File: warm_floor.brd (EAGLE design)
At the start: 52 x 40 mm, 31 parts, among them K1 G2R, Q1 BSS123, T1 BC847, T2 BC847, T3 BC847, X1 53047-04, X3 DG3XX-03-3.5, X4 DG3XX-02-3.5

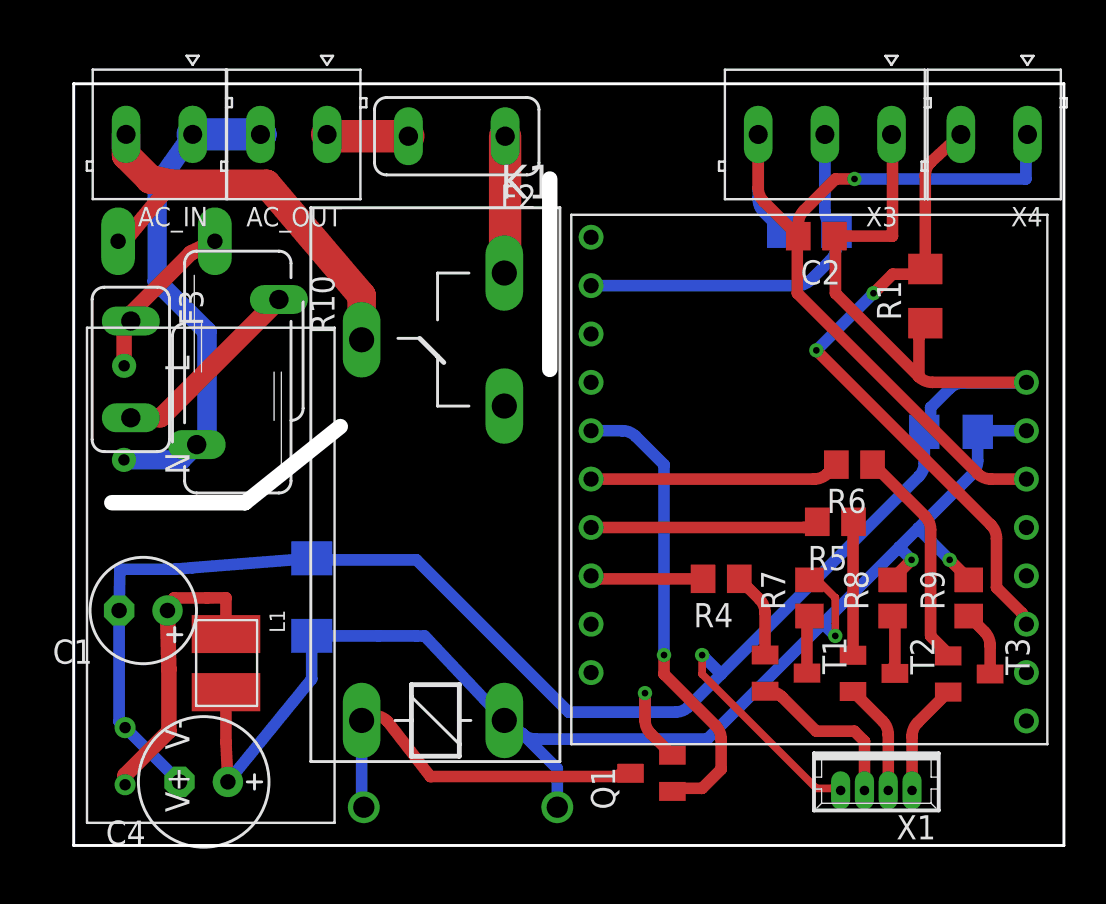
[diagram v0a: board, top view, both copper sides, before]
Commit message: Last G2R version
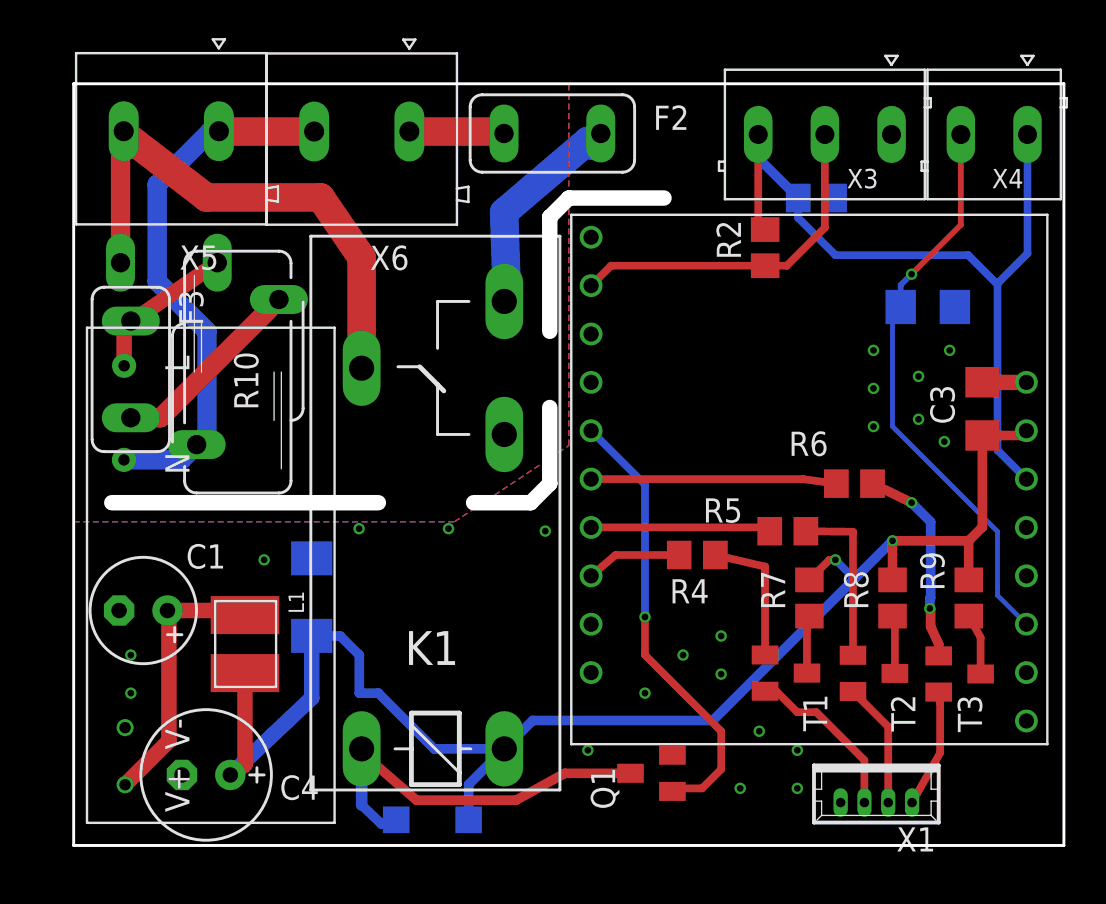
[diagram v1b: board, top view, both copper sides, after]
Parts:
- removed AC_IN, AC_OUT: DG3XX-02-3.5, degson:DG350-3.5-02P
- added X5, X6: DG3XX-025.0, degson:DG300-5.0-02P
- D1: value 1N4004 -> (none); device diode:DO41-10 -> diode:SOD123
- D2: value SMBJ20A -> SMBJ15A
- F1: value (none) -> FUSETE5; device fuse:TR5 -> fuse:TE5
- R2: device resistor:R1206 -> rcl:R0805
- moved F2 5.02 mm to (25.1, 37.4)
- moved R5 2.55 mm to (37.5, 16.5)
- moved R2 2.48 mm to (36.3, 31.4), flipped to the top, turned to 90 degrees
- moved C3 2.05 mm to (47.7, 22.9), flipped to the top, turned to 270 degrees
- moved C2 2.00 mm to (39.0, 34.0), flipped to the bottom, turned to 0 degrees
- moved R4 1.77 mm to (32.7, 15.3)
- moved D1 1.62 mm to (18.8, 1.35)
- moved K1 1.49 mm to (18.9, 7.61)
- moved L1 1.41 mm to (9.63, 10.8)
- moved F1 1.13 mm to (5.00, 30.6)
- moved R6 1.00 mm to (41.0, 19.0)
- moved X1 0.63 mm to (42.1, 2.71)
- moved R1 0.58 mm to (44.9, 28.3), flipped to the bottom, turned to 0 degrees
- moved T3 0.50 mm to (46.5, 9.01)
- moved C4 0.39 mm to (6.96, 3.71)
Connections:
- net L: now also X5.2; no longer AC_IN.2
- net N: now also X5.1, X6.2; no longer AC_IN.1, AC_OUT.2
- net WF_L: now also X6.1; no longer AC_OUT.1
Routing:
- net GND: track 115.4 -> 2.31 mm, vias 2 -> 22
- net 3.3V: track 47.5 -> 41.7 mm, vias 1 -> 0
- net RELAY_OUT: track 7.19 -> 11.6 mm
- net L: track 24.2 -> 28.2 mm
- net NTC: track 34.1 -> 30.1 mm, vias 2 -> 1
- net N$19: track 4.50 -> 7.32 mm
- net N$16: track 12.0 -> 9.44 mm
- net N: track 26.1 -> 28.6 mm
- net N$20: track 7.02 -> 8.96 mm
- net DATA: track 19.9 -> 18.4 mm
- net N$1: track 15.5 -> 14.4 mm
- net RELAY: track 24.7 -> 23.6 mm
- net N$22: track 5.91 -> 5.03 mm
- net PS_L: track 8.78 -> 7.99 mm
- net N$21: track 11.6 -> 10.9 mm, vias 0 -> 2
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- added copper zone on layer 1, net GND
- added copper zone on layer 16, net GND
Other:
- outline, holes or cut-outs redrawn
